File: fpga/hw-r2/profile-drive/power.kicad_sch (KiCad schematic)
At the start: 19 parts, among them J1 USB-C 16p, U5 TLV62568DBV 1V1, U6 TLV62568DBV 3V3, U7 TLV73325PDBV 2V5

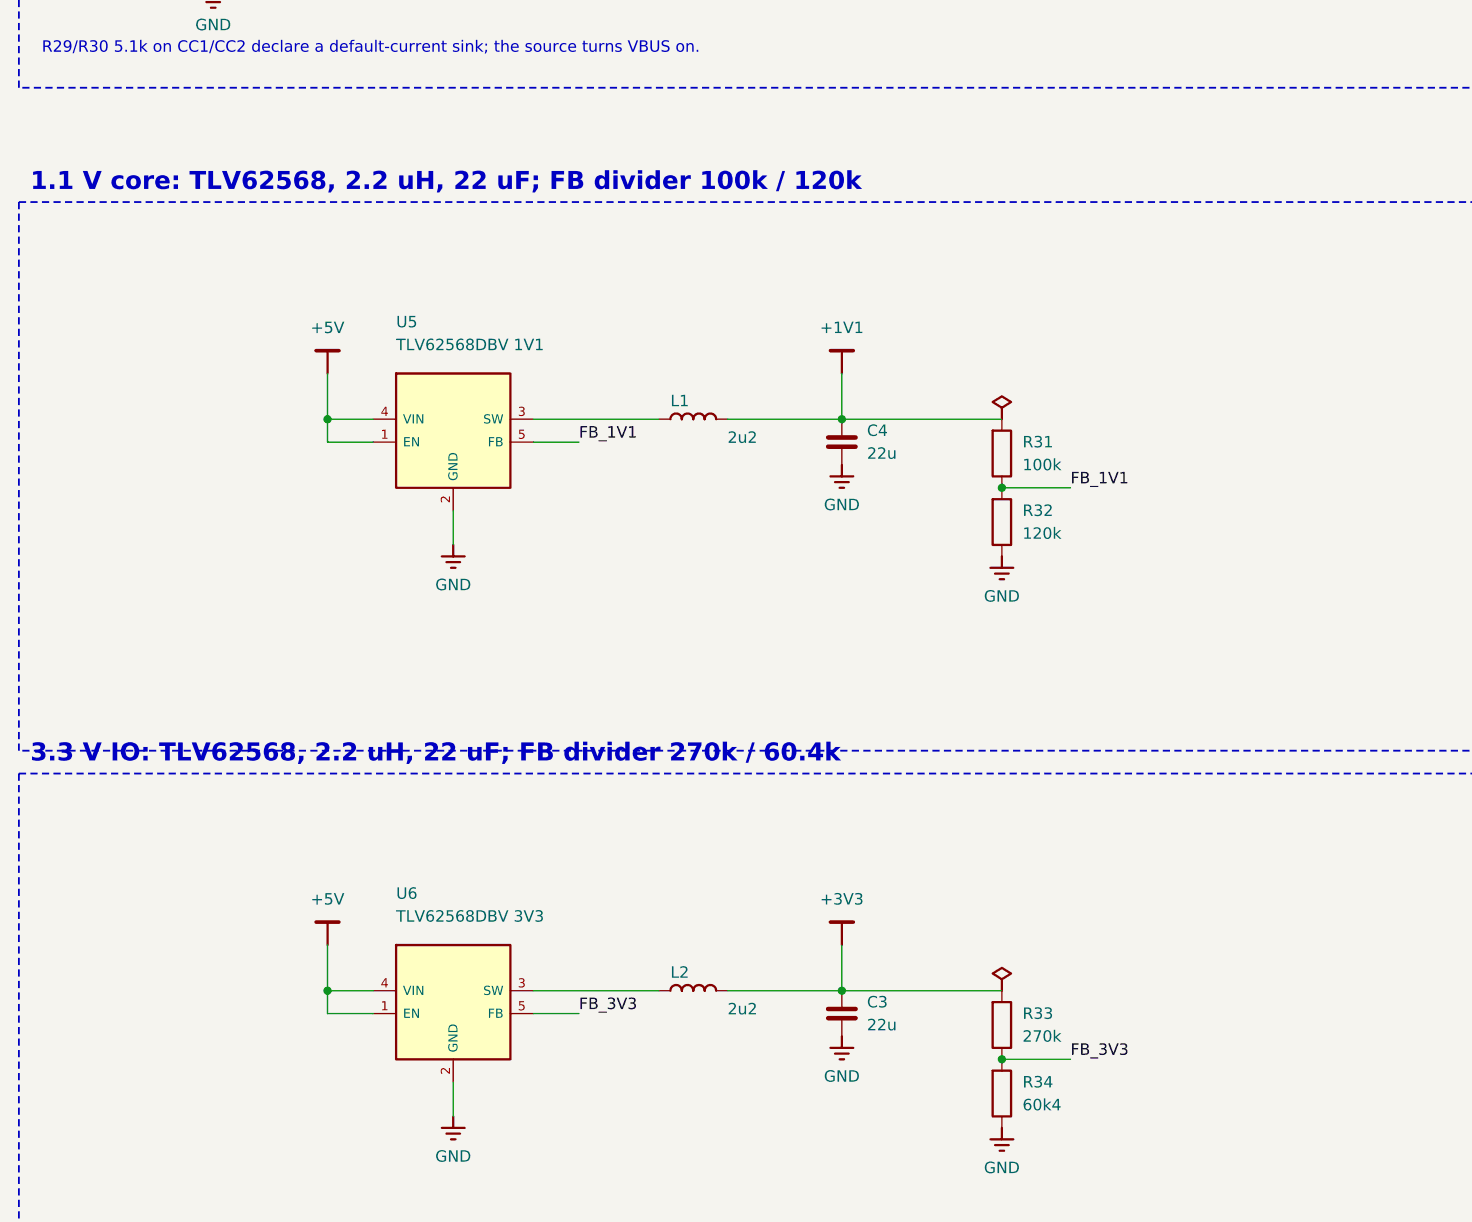
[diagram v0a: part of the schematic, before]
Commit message: fixups, tweaking
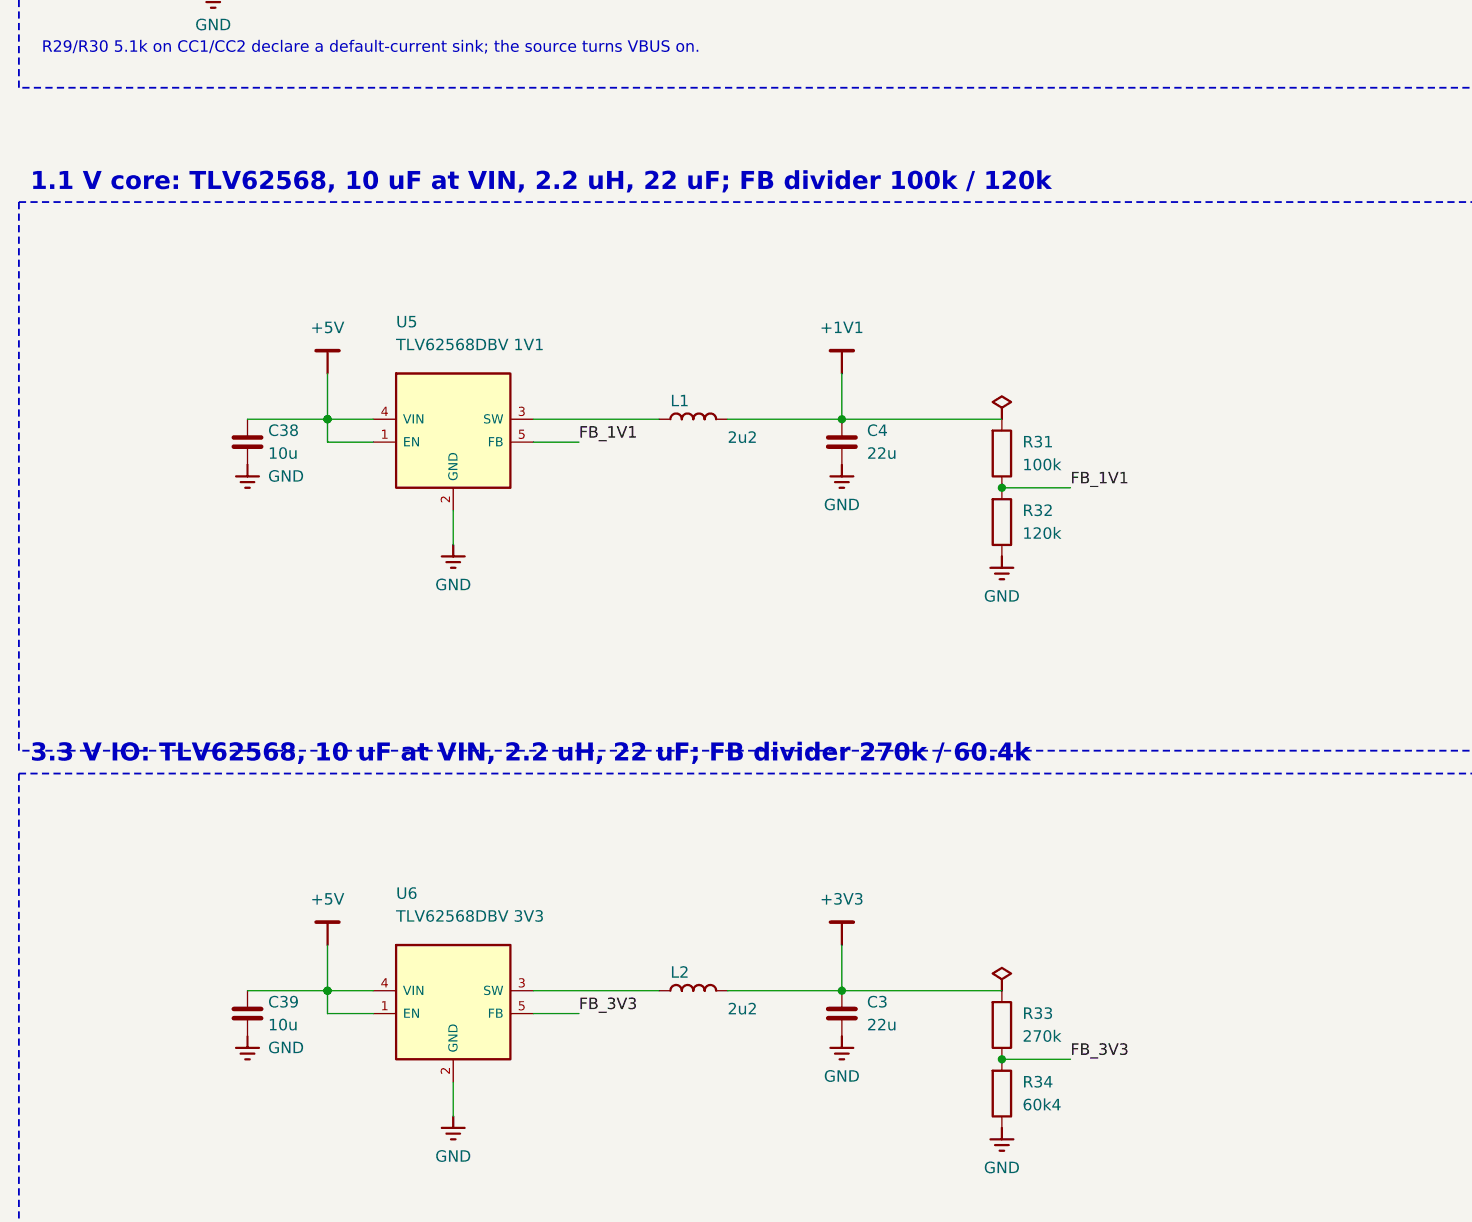
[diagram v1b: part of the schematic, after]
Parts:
- added C38, C39: 10u, Capacitor_SMD:C_0603_1608Metric, symbol device:C
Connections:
- net +5V: now also C38.1, C39.1
- net GND: now also C38.2, C39.2
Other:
- note added: "1.1 V core: TLV62568, 10 uF at VIN, 2.2 uH, 22 uF; FB divider 100k / 120k"
- note added: "3.3 V IO: TLV62568, 10 uF at VIN, 2.2 uH, 22 uF; FB divider 270k / 60.4k"
- note removed: "1.1 V core: TLV62568, 2.2 uH, 22 uF; FB divider 100k / 120k"
- note removed: "3.3 V IO: TLV62568, 2.2 uH, 22 uF; FB divider 270k / 60.4k"
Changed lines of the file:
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@@
   )
   (rectangle (start 15.24 114.3) (end 190.5 175.26) (stroke (width 0.2) (type dash)) (fill (type none)))
-  (text "1.1 V core: TLV62568, 2.2 uH, 22 uF; FB divider 100k / 120k" (exclude_from_sim no) (at 16.51 111 0) (effects (font (size 2 2) bold) (justify left top)))
+  (text "1.1 V core: TLV62568, 10 uF at VIN, 2.2 uH, 22 uF; FB divider 100k / 120k" (exclude_from_sim no) (at 16.51 111 0) (effects (font (size 2 2) bold) (justify left top)))
   (symbol (lib_id "device:TLV62568") (at 63.5 139.7 0) (unit 1)
     (exclude_from_sim no) (in_bom yes) (on_board yes) (dnp no)
@@
   (label "FB_1V1" (at 77.47 140.97 0) (fields_autoplaced yes) (effects (font (size 1.27 1.27)) (justify left bottom)))
   (rectangle (start 15.24 177.8) (end 190.5 238.76) (stroke (width 0.2) (type dash)) (fill (type none)))
-  (text "3.3 V IO: TLV62568, 2.2 uH, 22 uF; FB divider 270k / 60.4k" (exclude_from_sim no) (at 16.51 174.5 0) (effects (font (size 2 2) bold) (justify left top)))
+  (text "3.3 V IO: TLV62568, 10 uF at VIN, 2.2 uH, 22 uF; FB divider 270k / 60.4k" (exclude_from_sim no) (at 16.51 174.5 0) (effects (font (size 2 2) bold) (justify left top)))
   (symbol (lib_id "device:TLV62568") (at 63.5 203.2 0) (unit 1)
     (exclude_from_sim no) (in_bom yes) (on_board yes) (dnp no)
@@
   (text "Rails" (exclude_from_sim no) (at 203.2 38.1 0) (effects (font (size 2 2) bold) (justify left top)))
   (text "+5V       USB VBUS, bucks in\n+3V3      FPGA VCCIO, flash, oscillator, SD, 74LVC245 A side, LDO in\n+1V1      FPGA core\n+2V5      LDO output, only FB1 hangs on it\nVCCAUX_F  FPGA VCCAUX, after the ferrite\nGND       one plane" (exclude_from_sim no) (at 203.2 45.72 0) (effects (font (size 1.27 1.27)) (justify left top)))
+  (symbol (lib_id "device:C") (at 40.64 140.97 0) (unit 1)
+    (exclude_from_sim no) (in_bom yes) (on_board yes) (dnp no)
+    (property "Reference" "C38" (at 42.93 139.7 0) (effects (font (size 1.27 1.27)) (justify left)))
+    (property "Value" "10u" (at 42.93 142.24 0) (effects (font (size 1.27 1.27)) (justify left)))
+    (property "Footprint" "Capacitor_SMD:C_0603_1608Metric" (at 40.64 140.97 0) (effects (font (size 1.27 1.27)) hide))
+    (property "Datasheet" "" (at 40.64 140.97 0) (effects (font (size 1.27 1.27)) hide))
+    (property "Description" "capacitor" (at 40.64 140.97 0) (effects (font (size 1.27 1.27)) hide))
+    (pin "1")
+    (pin "2")
+    (instances (project "profile-drive" (path "/a55e218f-75e5-4ac7-a1a1-30827bd7ace5/52653336-3db4-5871-a322-379b0d9ed0e5" (reference "C38") (unit 1))))
+  )
+  (wire (pts (xy 40.64 138.43) (xy 49.53 138.43)) (stroke (width 0) (type default)))
+  (junction (at 49.53 138.43) (diameter 0) (color 0 0 0 0))
+  (symbol (lib_id "device:GND") (at 40.64 143.51 0) (unit 1)
+    (exclude_from_sim no) (in_bom no) (on_board yes) (dnp no)
+    (property "Reference" "#PWR903" (at 42.93 142.24 0) (effects (font (size 1.27 1.27)) hide))
+    (property "Value" "GND" (at 42.93 144.78 0) (effects (font (size 1.27 1.27)) (justify left)))
+    (property "Footprint" "" (at 40.64 143.51 0) (effects (font (size 1.27 1.27)) hide))
+    (property "Datasheet" "" (at 40.64 143.51 0) (effects (font (size 1.27 1.27)) hide))
+    (property "Description" "" (at 40.64 143.51 0) (effects (font (size 1.27 1.27)) hide))
+    (pin "1")
+    (instances (project "profile-drive" (path "/a55e218f-75e5-4ac7-a1a1-30827bd7ace5/52653336-3db4-5871-a322-379b0d9ed0e5" (reference "#PWR903") (unit 1))))
+  )
+  (symbol (lib_id "device:C") (at 40.64 204.47 0) (unit 1)
+    (exclude_from_sim no) (in_bom yes) (on_board yes) (dnp no)
+    (property "Reference" "C39" (at 42.93 203.2 0) (effects (font (size 1.27 1.27)) (justify left)))
+    (property "Value" "10u" (at 42.93 205.74 0) (effects (font (size 1.27 1.27)) (justify left)))
+    (property "Footprint" "Capacitor_SMD:C_0603_1608Metric" (at 40.64 204.47 0) (effects (font (size 1.27 1.27)) hide))
+    (property "Datasheet" "" (at 40.64 204.47 0) (effects (font (size 1.27 1.27)) hide))
+    (property "Description" "capacitor" (at 40.64 204.47 0) (effects (font (size 1.27 1.27)) hide))
+    (pin "1")
+    (pin "2")
+    (instances (project "profile-drive" (path "/a55e218f-75e5-4ac7-a1a1-30827bd7ace5/52653336-3db4-5871-a322-379b0d9ed0e5" (reference "C39") (unit 1))))
+  )
+  (wire (pts (xy 40.64 201.93) (xy 49.53 201.93)) (stroke (width 0) (type default)))
+  (junction (at 49.53 201.93) (diameter 0) (color 0 0 0 0))
+  (symbol (lib_id "device:GND") (at 40.64 207.01 0) (unit 1)
+    (exclude_from_sim no) (in_bom no) (on_board yes) (dnp no)
+    (property "Reference" "#PWR904" (at 42.93 205.74 0) (effects (font (size 1.27 1.27)) hide))
+    (property "Value" "GND" (at 42.93 208.28 0) (effects (font (size 1.27 1.27)) (justify left)))
+    (property "Footprint" "" (at 40.64 207.01 0) (effects (font (size 1.27 1.27)) hide))
+    (property "Datasheet" "" (at 40.64 207.01 0) (effects (font (size 1.27 1.27)) hide))
+    (property "Description" "" (at 40.64 207.01 0) (effects (font (size 1.27 1.27)) hide))
+    (pin "1")
+    (instances (project "profile-drive" (path "/a55e218f-75e5-4ac7-a1a1-30827bd7ace5/52653336-3db4-5871-a322-379b0d9ed0e5" (reference "#PWR904") (unit 1))))
+  )
   (sheet_instances (path "/" (page "2")))
 )
